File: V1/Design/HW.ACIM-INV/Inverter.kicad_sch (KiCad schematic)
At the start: 72 parts, among them J16 HIGH VOLTAGE OUTPUTS, J2 U, J3 V, J4 W, J5 N, J6 U, J7 V, J8 W, J9 N, M5 560V/1.75kA, M6 560V/1.75kA, M7 560V/1.75kA, Q3 20V/1A, U1 I=±10A, U10 DIGI ISO, U11 I=±10A, U12 I=±10A, U13 CMP-1CH, U7 IPM 600V/15A, U8 DIGI ISO, U9 DIGI ISO

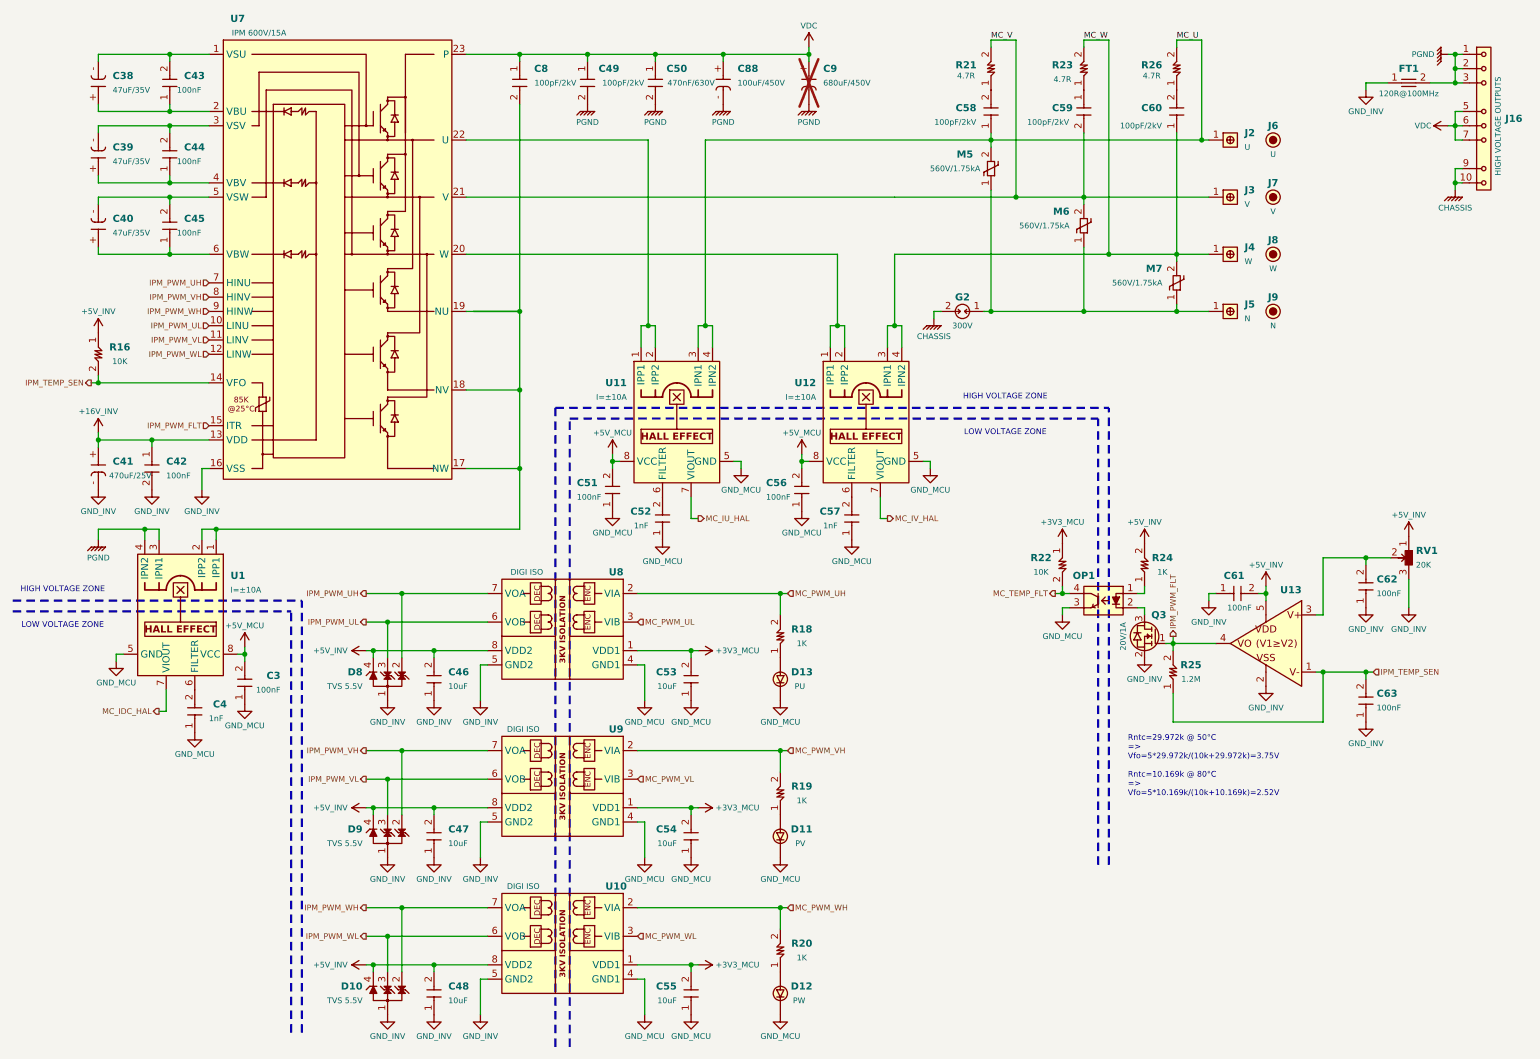
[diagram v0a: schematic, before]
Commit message: V1 schematic update 24
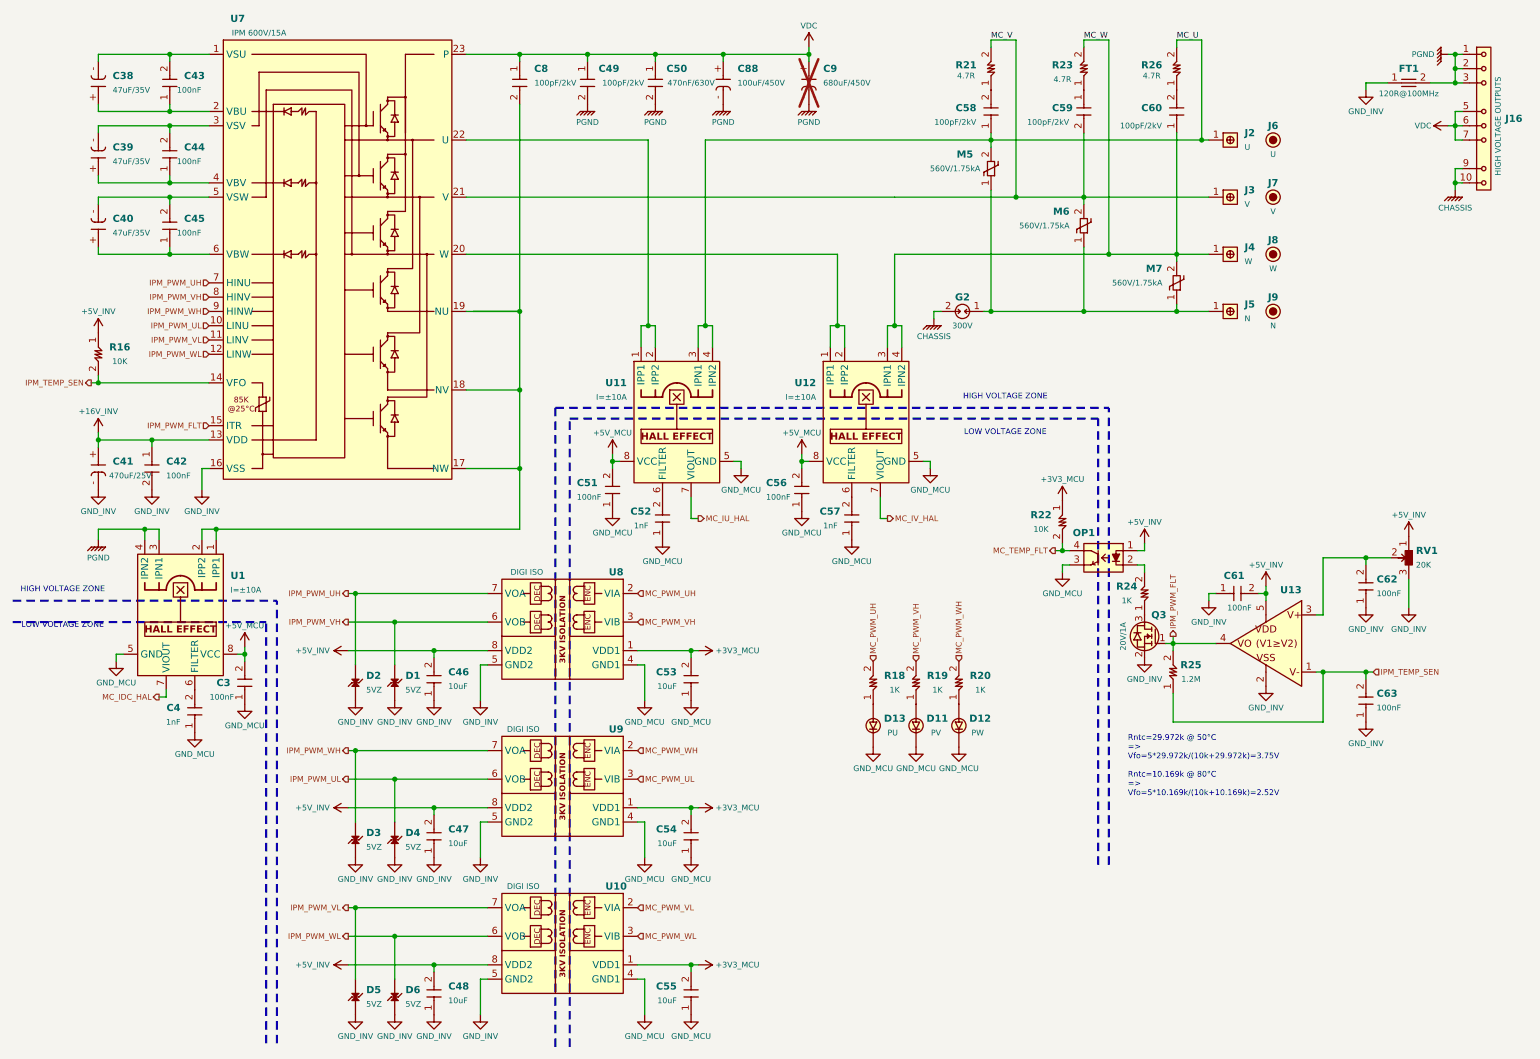
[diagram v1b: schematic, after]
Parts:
- removed D10, D8, D9: TVS 5.5V, SAMPI:SOT143B_NEXT, symbol SAM1:TVS_3CH
- added D1, D2, D3, D4, D5, D6: 5VZ, Liem:SOD-123FL_12, symbol SAMPI:TVS
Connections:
- net +5V_INV: now also OP1.1 (A); no longer R24.2
- net GND_INV: now also D1.2, D2.2, D3.2, D4.2, D5.2, D6.2
- net IPM_PWM_UH: now also D2.1
- net IPM_PWM_UL: now also U9.6 (VOB), D4.1; no longer U8.6 (VOB)
- net IPM_PWM_VH: now also U8.6 (VOB), D1.1; no longer U9.7 (VOA)
- net IPM_PWM_VL: now also U10.7 (VOA), D5.1; no longer U9.6 (VOB)
- net IPM_PWM_WH: now also U9.7 (VOA), D3.1; no longer U10.7 (VOA)
- net IPM_PWM_WL: now also D6.1
- net MC_PWM_UL: now also U9.3 (VIB); no longer U8.3 (VIB)
- net MC_PWM_VH: now also U8.3 (VIB); no longer U9.2 (VIA)
- net MC_PWM_VL: now also U10.2 (VIA); no longer U9.3 (VIB)
- net MC_PWM_WH: now also U9.2 (VIA); no longer U10.2 (VIA)
- net at R24.1: now also Q3.3 (D); no longer OP1.1 (A)
- net at OP1.2 (K): now also R24.2; no longer Q3.3 (D)
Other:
- moved on the sheet: D11, D12, D13, OP1, R18, R19, R20, R22, R24
